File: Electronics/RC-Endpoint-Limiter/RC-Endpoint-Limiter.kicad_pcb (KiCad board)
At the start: 2 copper layers, 46.8 x 29.9 mm, 58 parts, among them J1 USB_B_Micro, J10 ISCP, J11 POT Input, J2 Hall Low, J3 Hall High, J4 Switch Low, J5 Switch High, J6 RC Input, J7 RC Output, J8 Inhibit Input, J9 I²C header, U1 ATmega32U4-MU, Y1 8Mhz

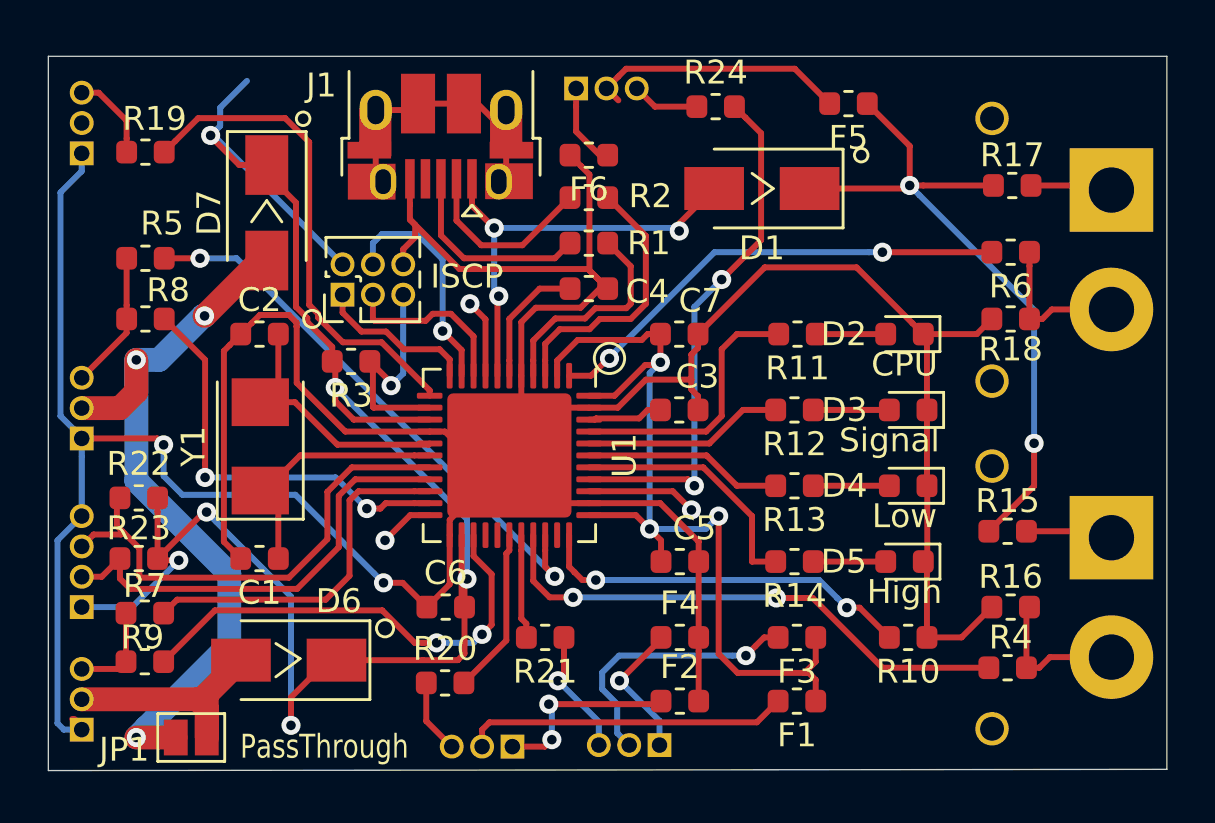
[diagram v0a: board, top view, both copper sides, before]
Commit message: polished up PCB layout
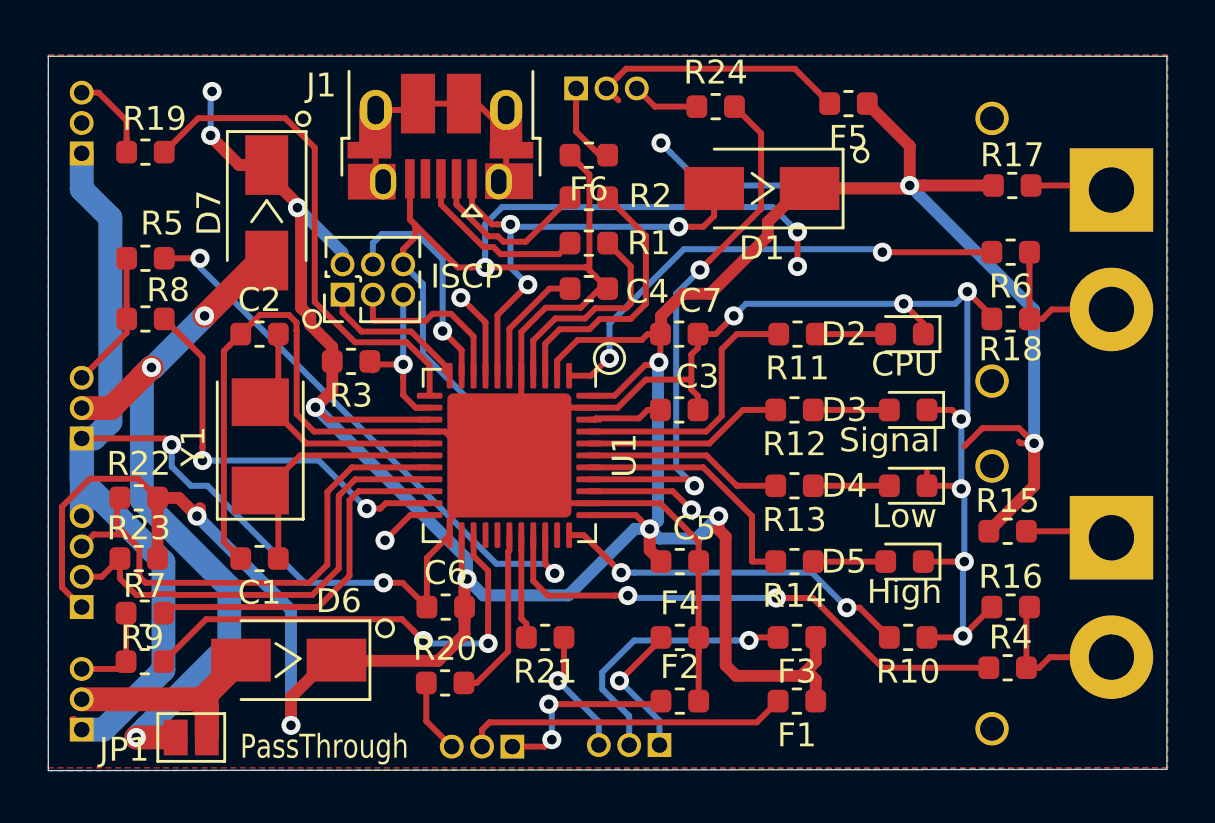
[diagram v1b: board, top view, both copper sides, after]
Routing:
- net GND: track 166.9 -> 204.6 mm, vias 2 -> 12
- net VCC: track 144.2 -> 176.8 mm, vias 11 -> 13
- net /RESET: track 9.33 -> 7.00 mm
- net Net-(D1-Pad2): track 18.9 -> 20.1 mm
- net Net-(D7-Pad2): track 31.8 -> 30.8 mm
- net Net-(R6-Pad2): track 19.8 -> 20.8 mm
- net Net-(J1-Pad3): track 8.43 -> 7.53 mm
- net Net-(J9-Pad3): track 20.9 -> 21.7 mm
- net Net-(R10-Pad2): track 16.0 -> 15.2 mm
- net Net-(J9-Pad2): track 19.1 -> 19.8 mm
- net Net-(R24-Pad2): track 22.0 -> 22.6 mm
- net Net-(J1-Pad2): track 7.76 -> 7.24 mm
- added copper zone on B.Cu, net GND
- added copper zone on F.Cu, net VCC
